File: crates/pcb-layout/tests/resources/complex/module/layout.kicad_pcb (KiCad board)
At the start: 2 copper layers, 4 parts

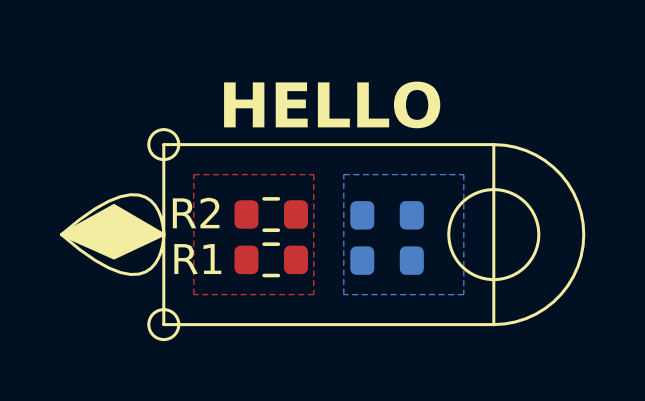
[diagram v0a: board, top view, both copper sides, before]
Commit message: sync vias and track
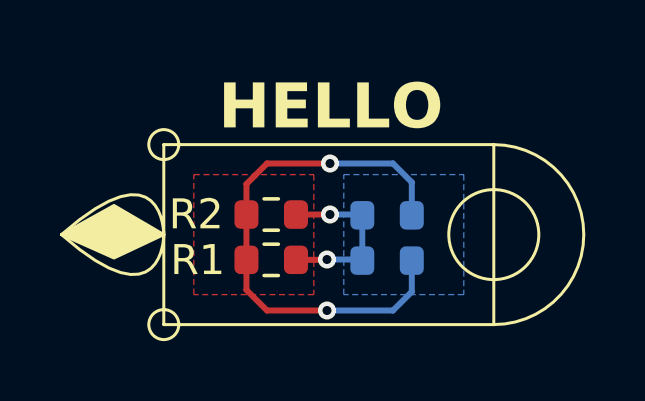
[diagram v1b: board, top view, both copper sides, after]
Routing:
- net P1: track 0.00 -> 17.8 mm, vias 0 -> 2
- net P2: track 0.00 -> 5.96 mm, vias 0 -> 2
